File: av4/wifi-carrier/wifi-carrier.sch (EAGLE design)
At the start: 13 parts, among them J1 ROCKETNET-CONNECTOR-16M, U1 UEI15

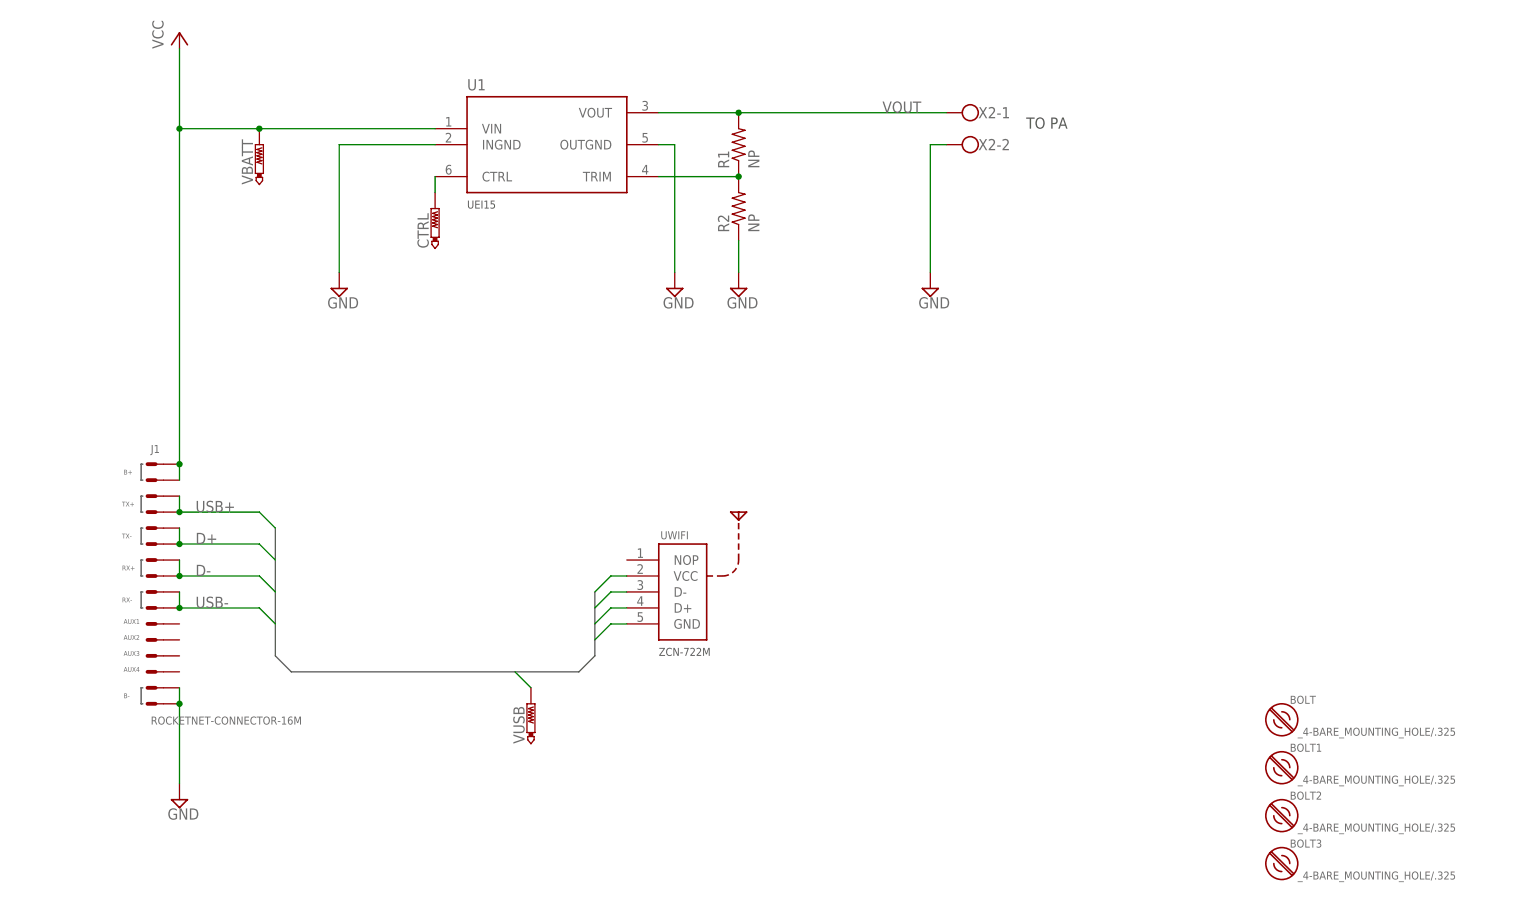
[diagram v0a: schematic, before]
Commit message: adding caps to wifi carrier
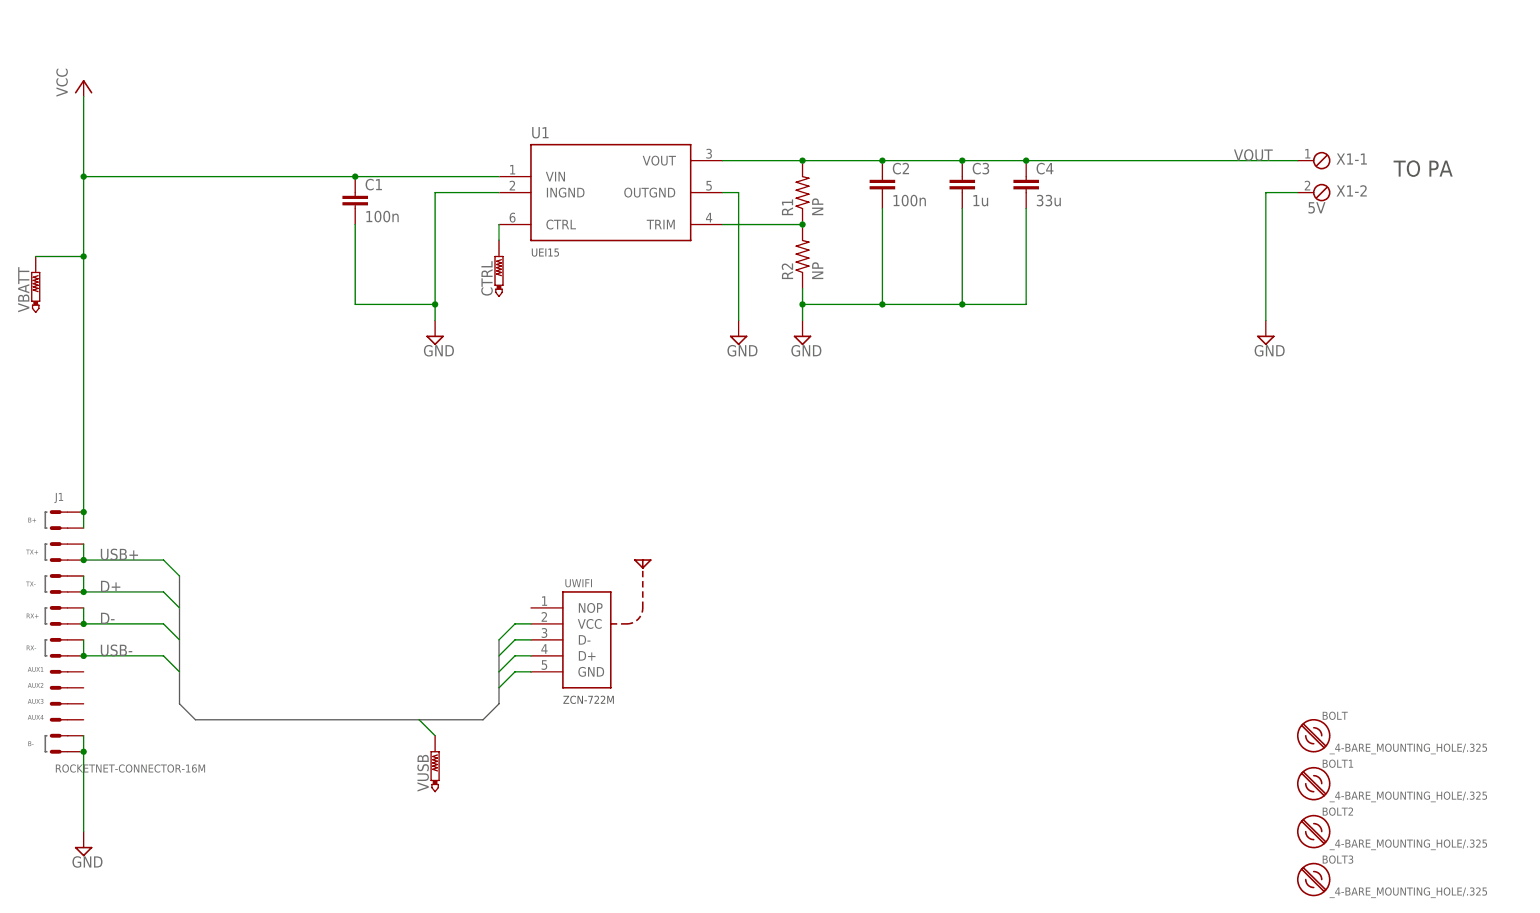
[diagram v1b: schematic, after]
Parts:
- removed X2: (no value), con-wago-500:W237-102
- added C1, C2: 100n, rcl:C-EUC0603
- added C3: 1u, rcl:C-EUC0805
- added C4: 33u, rcl:C-EUC1206
- added X1: 5V, con-phoenix-254:MPT2
- R1, R2: device rcl:R-US_R0805 -> rcl:R-US_R0603
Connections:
- net GND: now also C1.2, C2.2, C3.2, C4.2, X1-2.1; no longer X2-2.KL
- net VCC: now also C1.1
- net VOUT: now also C2.1, C3.1, C4.1, X1-1.1; no longer X2-1.KL
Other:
- moved on the sheet: BOLT, BOLT1, BOLT2, BOLT3, CTRL, J1, R1, R2, U1, UWIFI, VBATT, VUSB
